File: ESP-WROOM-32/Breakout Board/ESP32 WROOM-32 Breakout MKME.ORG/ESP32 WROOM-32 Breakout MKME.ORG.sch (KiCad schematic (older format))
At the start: 1 part, among them U1 ESP32_DevKit_V1_DOIT

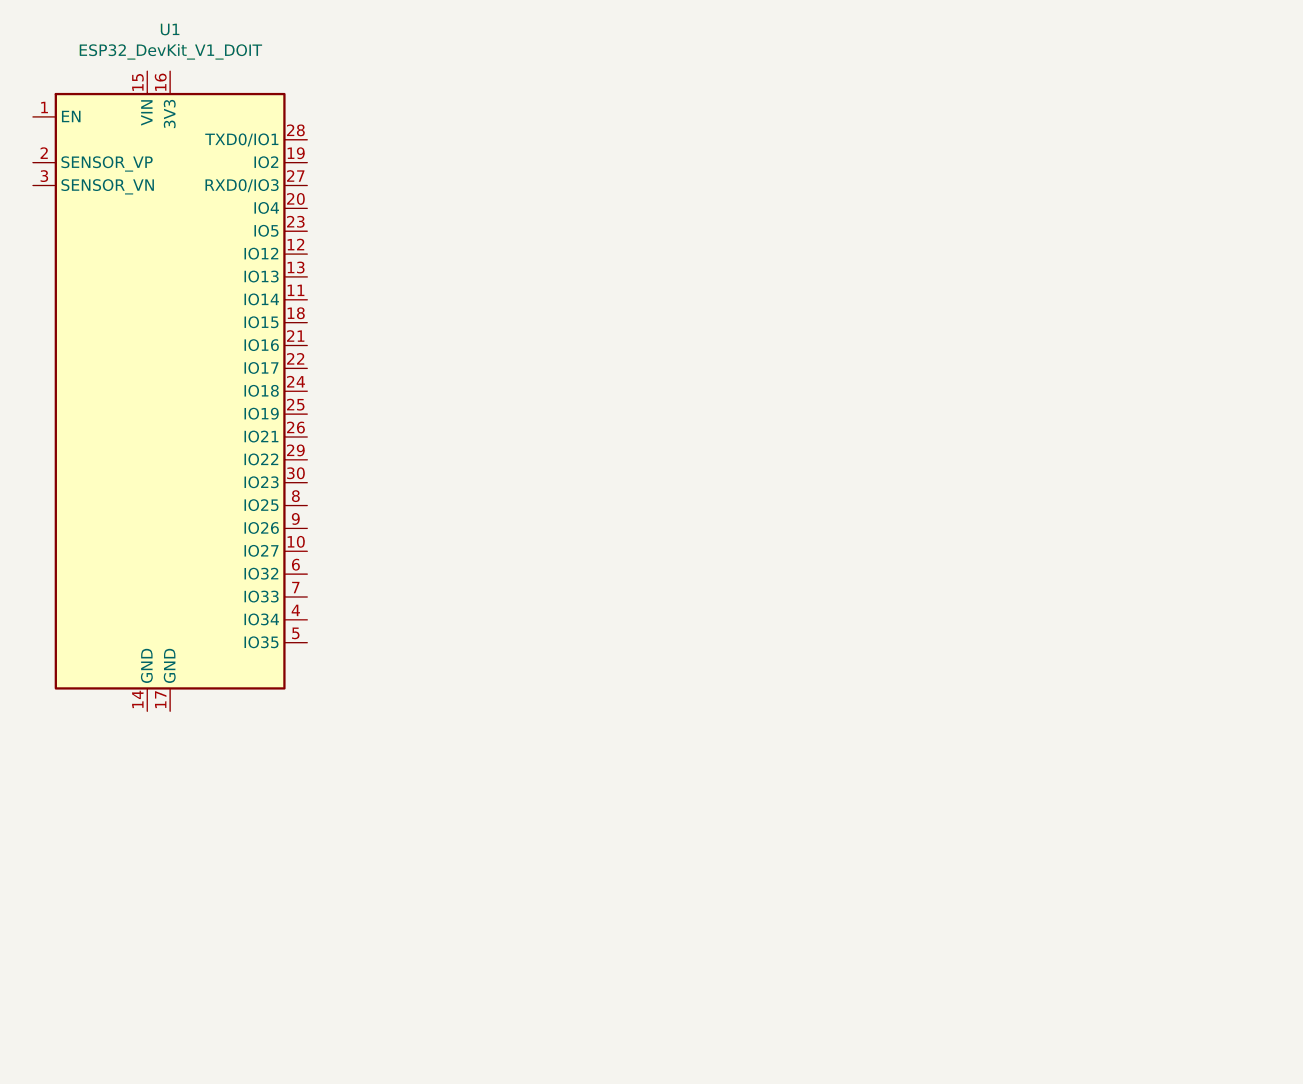
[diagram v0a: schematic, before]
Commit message: ref
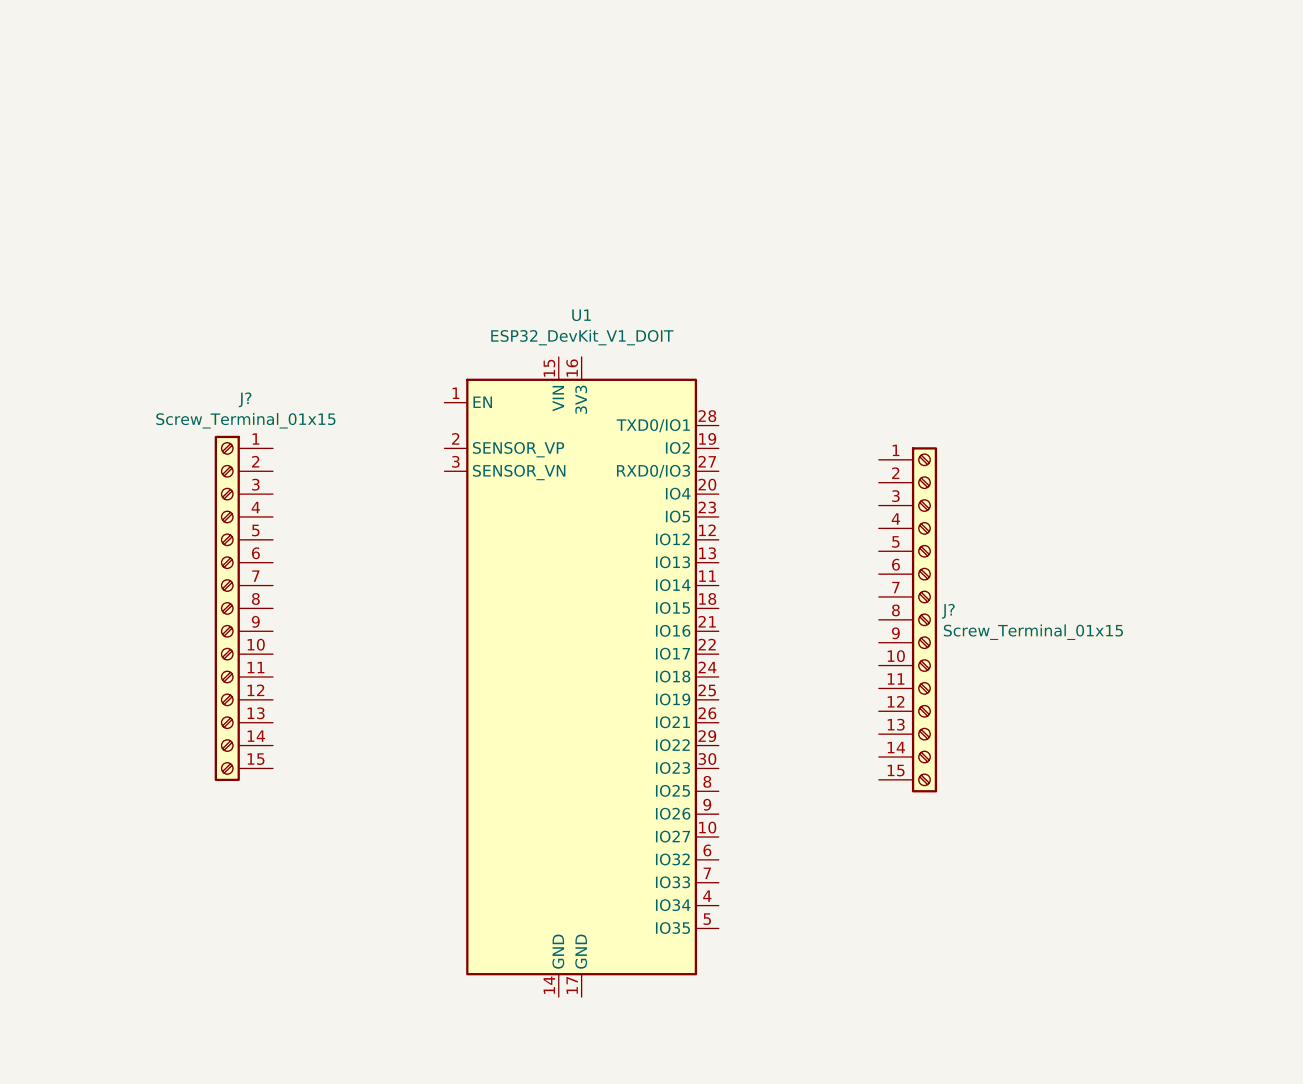
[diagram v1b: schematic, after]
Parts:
- added J? (x2): Screw_Terminal_01x15, symbol Connector:Screw_Terminal_01x15
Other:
- moved on the sheet: U1
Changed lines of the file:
@@
 L ESp3222:ESP32_DevKit_V1_DOIT U1
 U 1 1 6134E7FD
-P 6450 3350
-F 0 "U1" H 6450 4931 50  0000 C CNN
-F 1 "ESP32_DevKit_V1_DOIT" H 6450 4840 50  0000 C CNN
-F 2 "esp322:esp32_devkit_v1_doit" H 6000 4700 50  0001 C CNN
-F 3 "https://aliexpress.com/item/32864722159.html" H 6000 4700 50  0001 C CNN
-	1    6450 3350
+P 8250 4600
+F 0 "U1" H 8250 6181 50  0000 C CNN
+F 1 "ESP32_DevKit_V1_DOIT" H 8250 6090 50  0000 C CNN
+F 2 "esp322:esp32_devkit_v1_doit" H 7800 5950 50  0001 C CNN
+F 3 "https://aliexpress.com/item/32864722159.html" H 7800 5950 50  0001 C CNN
+	1    8250 4600
 	1    0    0    -1
 $EndComp
+$Comp
+L Connector:Screw_Terminal_01x15 J?
+U 1 1 61353EE6
+P 9750 4350
+F 0 "J?" H 9830 4392 50  0000 L CNN
+F 1 "Screw_Terminal_01x15" H 9830 4301 50  0000 L CNN
+F 2 "" H 9750 4350 50  0001 C CNN
+F 3 "~" H 9750 4350 50  0001 C CNN
+	1    9750 4350
+	1    0    0    -1
+$EndComp
+$Comp
+L Connector:Screw_Terminal_01x15 J?
+U 1 1 61354F94
+P 6700 4300
+F 0 "J?" H 6618 5217 50  0000 C CNN
+F 1 "Screw_Terminal_01x15" H 6618 5126 50  0000 C CNN
+F 2 "" H 6700 4300 50  0001 C CNN
+F 3 "~" H 6700 4300 50  0001 C CNN
+	1    6700 4300
+	-1   0    0    -1
+$EndComp
 $EndSCHEMATC

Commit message: Photos and kit updated
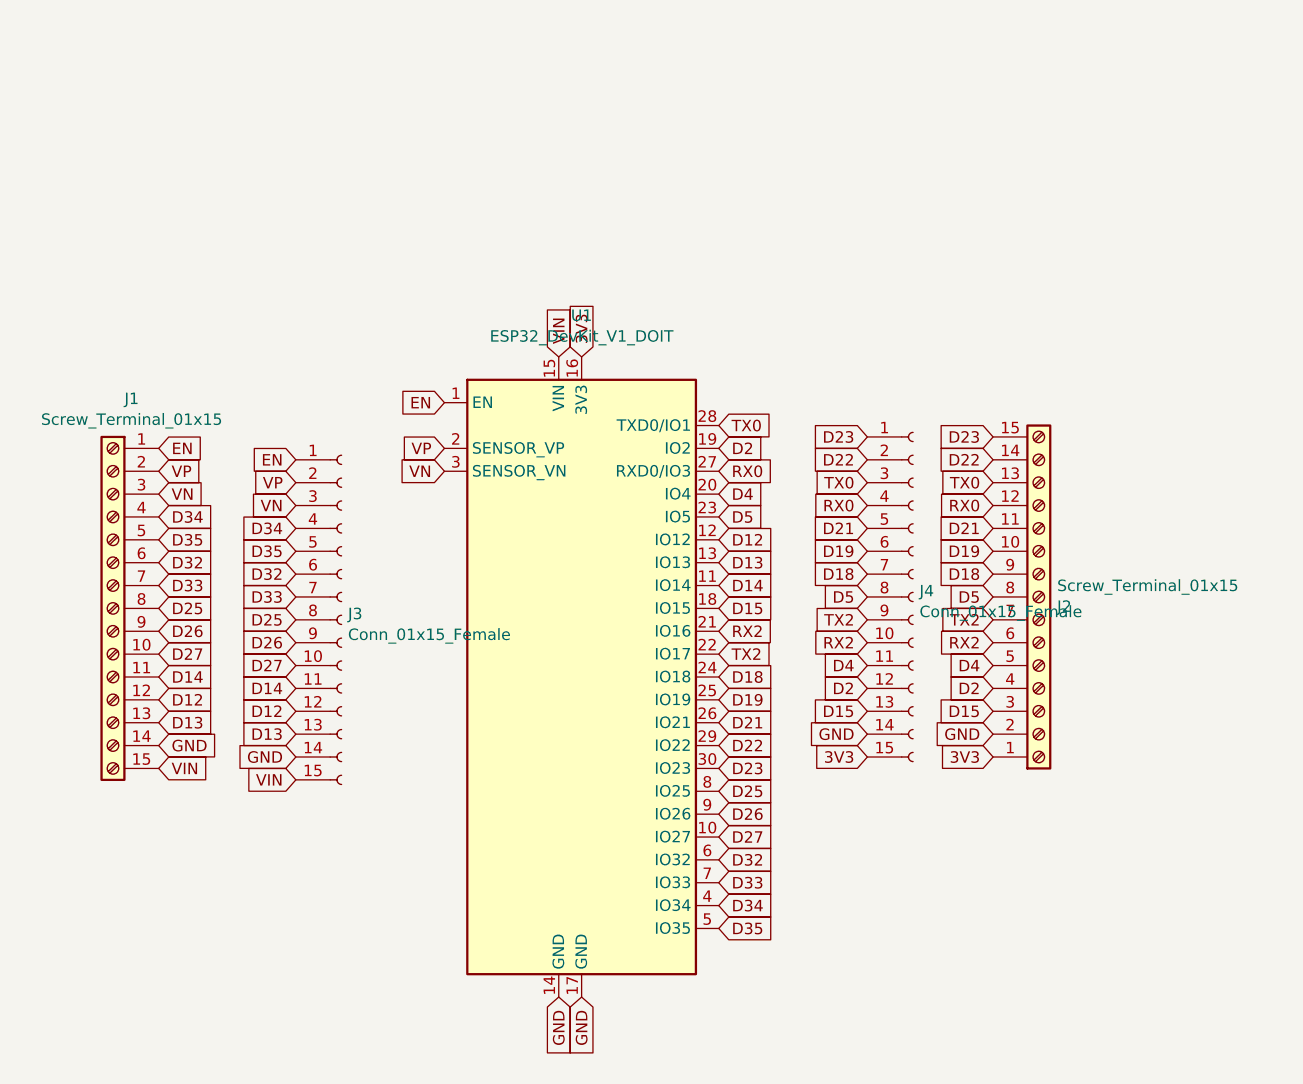
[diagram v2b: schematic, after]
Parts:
- added J3, J4: Conn_01x15_Female, Connector_PinHeader_2.54mm:PinHeader_1x15_P2.54mm_Vertical, symbol Connector:Conn_01x15_Female
- J1, J2: renamed from J?; footprint (none) -> TerminalBlock_Phoenix:TerminalBlock_Phoenix_MKDS-1,5-15-5.08_1x15_P5.08mm_Horizontal
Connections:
- net EN: now reaches U1.1 (EN)
- net EN: now also J1.1 (Pin_1), J3.1 (Pin_1)
- net D27: now reaches U1.10 (IO27)
- net D27: now also J1.10 (Pin_10), J3.10 (Pin_10)
- net D14: now reaches U1.11 (IO14)
- net D14: now also J1.11 (Pin_11), J3.11 (Pin_11)
- net D12: now reaches U1.12 (IO12)
- net D12: now also J1.12 (Pin_12), J3.12 (Pin_12)
- net D13: now reaches U1.13 (IO13)
- net D13: now also J1.13 (Pin_13), J3.13 (Pin_13)
- net GND: now reaches U1.14 (GND)
- net GND: now also J1.14 (Pin_14), J2.2 (Pin_2), U1.17 (GND), J3.14 (Pin_14), J4.14 (Pin_14)
- net VIN: now reaches U1.15 (VIN)
- net VIN: now also J1.15 (Pin_15), J3.15 (Pin_15)
- net 3V3: now reaches U1.16 (3V3)
- net 3V3: now also J2.1 (Pin_1), J4.15 (Pin_15)
- net D15: now reaches U1.18 (IO15)
- net D15: now also J2.3 (Pin_3), J4.13 (Pin_13)
- net D2: now reaches U1.19 (IO2)
- net D2: now also J2.4 (Pin_4), J4.12 (Pin_12)
- net VP: now reaches U1.2 (SENSOR_VP)
- net VP: now also J1.2 (Pin_2), J3.2 (Pin_2)
- net D4: now reaches U1.20 (IO4)
- net D4: now also J2.5 (Pin_5), J4.11 (Pin_11)
- net RX2: now reaches U1.21 (IO16)
- net RX2: now also J2.6 (Pin_6), J4.10 (Pin_10)
- net TX2: now reaches U1.22 (IO17)
- net TX2: now also J2.7 (Pin_7), J4.9 (Pin_9)
- net D5: now reaches U1.23 (IO5)
- net D5: now also J2.8 (Pin_8), J4.8 (Pin_8)
- net D18: now reaches U1.24 (IO18)
- net D18: now also J2.9 (Pin_9), J4.7 (Pin_7)
- net D19: now reaches U1.25 (IO19)
- net D19: now also J2.10 (Pin_10), J4.6 (Pin_6)
- net D21: now reaches U1.26 (IO21)
- net D21: now also J2.11 (Pin_11), J4.5 (Pin_5)
- net RX0: now reaches U1.27 (RXD0/IO3)
- net RX0: now also J2.12 (Pin_12), J4.4 (Pin_4)
- net TX0: now reaches U1.28 (TXD0/IO1)
- net TX0: now also J2.13 (Pin_13), J4.3 (Pin_3)
- net D22: now reaches U1.29 (IO22)
- net D22: now also J2.14 (Pin_14), J4.2 (Pin_2)
- net VN: now reaches U1.3 (SENSOR_VN)
- net VN: now also J1.3 (Pin_3), J3.3 (Pin_3)
- net D23: now reaches U1.30 (IO23)
- net D23: now also J2.15 (Pin_15), J4.1 (Pin_1)
- net D34: now reaches U1.4 (IO34)
- net D34: now also J1.4 (Pin_4), J3.4 (Pin_4)
- net D35: now reaches U1.5 (IO35)
- net D35: now also J1.5 (Pin_5), J3.5 (Pin_5)
- net D32: now reaches U1.6 (IO32)
- net D32: now also J1.6 (Pin_6), J3.6 (Pin_6)
- net D33: now reaches U1.7 (IO33)
- net D33: now also J1.7 (Pin_7), J3.7 (Pin_7)
- net D25: now reaches U1.8 (IO25)
- net D25: now also J1.8 (Pin_8), J3.8 (Pin_8)
- net D26: now reaches U1.9 (IO26)
- net D26: now also J1.9 (Pin_9), J3.9 (Pin_9)
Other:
- moved on the sheet: J1, J2
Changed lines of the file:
@@
 $EndDescr
+$Comp
+L Connector:Screw_Terminal_01x15 J2
+U 1 1 61353EE6
+P 10250 4250
+F 0 "J2" H 10330 4292 50  0000 L CNN
+F 1 "Screw_Terminal_01x15" H 10330 4201 50  0000 L CNN
+F 2 "TerminalBlock_Phoenix:TerminalBlock_Phoenix_MKDS-1,5-15-5.08_1x15_P5.08mm_Horizontal" H 10250 4250 50  0001 C CNN
+F 3 "~" H 10250 4250 50  0001 C CNN
+	1    10250 4250
+	1    0    0    1
+$EndComp
+$Comp
+L Connector:Screw_Terminal_01x15 J1
+U 1 1 61354F94
+P 6200 4300
+F 0 "J1" H 6118 5217 50  0000 C CNN
+F 1 "Screw_Terminal_01x15" H 6118 5126 50  0000 C CNN
+F 2 "TerminalBlock_Phoenix:TerminalBlock_Phoenix_MKDS-1,5-15-5.08_1x15_P5.08mm_Horizontal" H 6200 4300 50  0001 C CNN
+F 3 "~" H 6200 4300 50  0001 C CNN
+	1    6200 4300
+	-1   0    0    -1
+$EndComp
+Text GLabel 6400 3600 2    50   Input ~ 0
+EN
+Text GLabel 6400 3700 2    50   Input ~ 0
+VP
+Text GLabel 6400 4000 2    50   Input ~ 0
+D35
+Text GLabel 6400 3900 2    50   Input ~ 0
+D34
+Text GLabel 6400 4100 2    50   Input ~ 0
+D32
+Text GLabel 6400 4200 2    50   Input ~ 0
+D33
+Text GLabel 6400 4300 2    50   Input ~ 0
+D25
+Text GLabel 6400 4400 2    50   Input ~ 0
+D26
+Text GLabel 6400 4500 2    50   Input ~ 0
+D27
+Text GLabel 6400 4600 2    50   Input ~ 0
+D14
+Text GLabel 6400 4700 2    50   Input ~ 0
+D12
+Text GLabel 6400 4800 2    50   Input ~ 0
+D13
+Text GLabel 6400 4900 2    50   Input ~ 0
+GND
+Text GLabel 6400 5000 2    50   Input ~ 0
+VIN
+Text GLabel 6400 3800 2    50   Input ~ 0
+VN
+Text GLabel 7650 3400 0    50   Input ~ 0
+EN
+Text GLabel 8850 5700 2    50   Input ~ 0
+D35
+Text GLabel 8850 5600 2    50   Input ~ 0
+D34
+Text GLabel 8850 5400 2    50   Input ~ 0
+D32
+Text GLabel 8850 5500 2    50   Input ~ 0
+D33
+Text GLabel 8850 5100 2    50   Input ~ 0
+D25
+Text GLabel 8850 5200 2    50   Input ~ 0
+D26
+Text GLabel 8850 5300 2    50   Input ~ 0
+D27
+Text GLabel 8850 4200 2    50   Input ~ 0
+D14
+Text GLabel 8850 4000 2    50   Input ~ 0
+D12
+Text GLabel 8850 4100 2    50   Input ~ 0
+D13
+Text GLabel 8150 6000 3    50   Input ~ 0
+GND
+Text GLabel 8150 3200 1    50   Input ~ 0
+VIN
+Text GLabel 7650 3700 0    50   Input ~ 0
+VN
+Text GLabel 10050 3550 0    50   Input ~ 0
+D23
+Text GLabel 10050 3650 0    50   Input ~ 0
+D22
+Text GLabel 10050 3750 0    50   Input ~ 0
+TX0
+Text GLabel 10050 3850 0    50   Input ~ 0
+RX0
+Text GLabel 10050 3950 0    50   Input ~ 0
+D21
+Text GLabel 10050 4050 0    50   Input ~ 0
+D19
+Text GLabel 10050 4150 0    50   Input ~ 0
+D18
+Text GLabel 10050 4250 0    50   Input ~ 0
+D5
+Text GLabel 10050 4350 0    50   Input ~ 0
+TX2
+Text GLabel 10050 4450 0    50   Input ~ 0
+RX2
+Text GLabel 10050 4550 0    50   Input ~ 0
+D4
+Text GLabel 10050 4650 0    50   Input ~ 0
+D2
+Text GLabel 10050 4750 0    50   Input ~ 0
+D15
+Text GLabel 10050 4850 0    50   Input ~ 0
+GND
+Text GLabel 10050 4950 0    50   Input ~ 0
+3V3
+Text GLabel 8850 5000 2    50   Input ~ 0
+D23
+Text GLabel 8850 4900 2    50   Input ~ 0
+D22
+Text GLabel 8850 3500 2    50   Input ~ 0
+TX0
+Text GLabel 8850 3700 2    50   Input ~ 0
+RX0
+Text GLabel 8850 4800 2    50   Input ~ 0
+D21
+Text GLabel 8850 4700 2    50   Input ~ 0
+D19
+Text GLabel 8850 4600 2    50   Input ~ 0
+D18
+Text GLabel 8850 3900 2    50   Input ~ 0
+D5
+Text GLabel 8850 4500 2    50   Input ~ 0
+TX2
+Text GLabel 8850 4400 2    50   Input ~ 0
+RX2
+Text GLabel 8850 3800 2    50   Input ~ 0
+D4
+Text GLabel 8850 3600 2    50   Input ~ 0
+D2
+Text GLabel 8850 4300 2    50   Input ~ 0
+D15
+Text GLabel 8250 6000 3    50   Input ~ 0
+GND
+Text GLabel 8250 3200 1    50   Input ~ 0
+3V3
+Text GLabel 7650 3600 0    50   Input ~ 0
+VP
 $Comp
 L ESp3222:ESP32_DevKit_V1_DOIT U1
@@
 $EndComp
 $Comp
-L Connector:Screw_Terminal_01x15 J?
-U 1 1 61353EE6
-P 9750 4350
-F 0 "J?" H 9830 4392 50  0000 L CNN
-F 1 "Screw_Terminal_01x15" H 9830 4301 50  0000 L CNN
-F 2 "" H 9750 4350 50  0001 C CNN
-F 3 "~" H 9750 4350 50  0001 C CNN
-	1    9750 4350
+L Connector:Conn_01x15_Female J3
+U 1 1 615E00ED
+P 7200 4350
+F 0 "J3" H 7228 4376 50  0000 L CNN
+F 1 "Conn_01x15_Female" H 7228 4285 50  0000 L CNN
+F 2 "Connector_PinHeader_2.54mm:PinHeader_1x15_P2.54mm_Vertical" H 7200 4350 50  0001 C CNN
+F 3 "~" H 7200 4350 50  0001 C CNN
+	1    7200 4350
 	1    0    0    -1
 $EndComp
 $Comp
-L Connector:Screw_Terminal_01x15 J?
-U 1 1 61354F94
-P 6700 4300
-F 0 "J?" H 6618 5217 50  0000 C CNN
-F 1 "Screw_Terminal_01x15" H 6618 5126 50  0000 C CNN
-F 2 "" H 6700 4300 50  0001 C CNN
-F 3 "~" H 6700 4300 50  0001 C CNN
-	1    6700 4300
-	-1   0    0    -1
-$EndComp
+L Connector:Conn_01x15_Female J4
+U 1 1 615E1469
+P 9700 4250
+F 0 "J4" H 9728 4276 50  0000 L CNN
+F 1 "Conn_01x15_Female" H 9728 4185 50  0000 L CNN
+F 2 "Connector_PinHeader_2.54mm:PinHeader_1x15_P2.54mm_Vertical" H 9700 4250 50  0001 C CNN
+F 3 "~" H 9700 4250 50  0001 C CNN
+	1    9700 4250
+	1    0    0    -1
+$EndComp
+Text GLabel 7000 4950 0    50   Input ~ 0
+GND
+Text GLabel 7000 5050 0    50   Input ~ 0
+VIN
+Text GLabel 7000 3850 0    50   Input ~ 0
+VN
+Text GLabel 7000 4850 0    50   Input ~ 0
+D13
+Text GLabel 7000 4750 0    50   Input ~ 0
+D12
+Text GLabel 7000 4650 0    50   Input ~ 0
+D14
+Text GLabel 7000 4550 0    50   Input ~ 0
+D27
+Text GLabel 7000 4450 0    50   Input ~ 0
+D26
+Text GLabel 7000 4350 0    50   Input ~ 0
+D25
+Text GLabel 7000 4250 0    50   Input ~ 0
+D33
+Text GLabel 7000 4150 0    50   Input ~ 0
+D32
+Text GLabel 7000 3950 0    50   Input ~ 0
+D34
+Text GLabel 7000 4050 0    50   Input ~ 0
+D35
+Text GLabel 7000 3750 0    50   Input ~ 0
+VP
+Text GLabel 7000 3650 0    50   Input ~ 0
+EN
+Text GLabel 9500 3550 0    50   Input ~ 0
+D23
+Text GLabel 9500 3650 0    50   Input ~ 0
+D22
+Text GLabel 9500 3750 0    50   Input ~ 0
+TX0
+Text GLabel 9500 3850 0    50   Input ~ 0
+RX0
+Text GLabel 9500 3950 0    50   Input ~ 0
+D21
+Text GLabel 9500 4050 0    50   Input ~ 0
+D19
+Text GLabel 9500 4150 0    50   Input ~ 0
+D18
+Text GLabel 9500 4250 0    50   Input ~ 0
+D5
+Text GLabel 9500 4350 0    50   Input ~ 0
+TX2
+Text GLabel 9500 4450 0    50   Input ~ 0
+RX2
+Text GLabel 9500 4550 0    50   Input ~ 0
+D4
+Text GLabel 9500 4650 0    50   Input ~ 0
+D2
+Text GLabel 9500 4750 0    50   Input ~ 0
+D15
+Text GLabel 9500 4850 0    50   Input ~ 0
+GND
+Text GLabel 9500 4950 0    50   Input ~ 0
+3V3
 $EndSCHEMATC

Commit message: Breakout board DONE
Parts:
- J1: footprint TerminalBlock_Phoenix:TerminalBlock_Phoenix_MKDS-1,5-15-5.08_1x15_P5.08mm_Horizontal -> TerminalBlock_Phoenix:TerminalBlock_Phoenix_MKDS-1,5-16-5.08_1x16_P5.08mm_Horizontal
- J2: footprint TerminalBlock_Phoenix:TerminalBlock_Phoenix_MKDS-1,5-15-5.08_1x15_P5.08mm_Horizontal -> TerminalBlock_Phoenix:TerminalBlock_Phoenix_MKDS-1,5-16-5.08_1x16_P5.08mm_Horizontal; symbol Connector:Screw_Terminal_01x15 -> Connector:Screw_Terminal_01x16
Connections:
- net 3V3: now also J2.2 (Pin_2); no longer J2.1 (Pin_1)
- net D15: now also J2.4 (Pin_4); no longer J2.3 (Pin_3)
- net D18: now also J2.10 (Pin_10); no longer J2.9 (Pin_9)
- net D19: now also J2.11 (Pin_11); no longer J2.10 (Pin_10)
- net D2: now also J2.5 (Pin_5); no longer J2.4 (Pin_4)
- net D21: now also J2.12 (Pin_12); no longer J2.11 (Pin_11)
- net D22: now also J2.15 (Pin_15); no longer J2.14 (Pin_14)
- net D23: now also J2.16 (Pin_16); no longer J2.15 (Pin_15)
- net D4: now also J2.6 (Pin_6); no longer J2.5 (Pin_5)
- net D5: now also J2.9 (Pin_9); no longer J2.8 (Pin_8)
- net GND: now also J2.3 (Pin_3); no longer J2.2 (Pin_2)
- net RX0: now also J2.13 (Pin_13); no longer J2.12 (Pin_12)
- net RX2: now also J2.7 (Pin_7); no longer J2.6 (Pin_6)
- net TX0: now also J2.14 (Pin_14); no longer J2.13 (Pin_13)
- net TX2: now also J2.8 (Pin_8); no longer J2.7 (Pin_7)
- no-connect marks 0 -> 1
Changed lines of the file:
@@
 $EndDescr
-$Comp
-L Connector:Screw_Terminal_01x15 J2
-U 1 1 61353EE6
-P 10250 4250
-F 0 "J2" H 10330 4292 50  0000 L CNN
-F 1 "Screw_Terminal_01x15" H 10330 4201 50  0000 L CNN
-F 2 "TerminalBlock_Phoenix:TerminalBlock_Phoenix_MKDS-1,5-15-5.08_1x15_P5.08mm_Horizontal" H 10250 4250 50  0001 C CNN
-F 3 "~" H 10250 4250 50  0001 C CNN
-	1    10250 4250
-	1    0    0    1
-$EndComp
 $Comp
 L Connector:Screw_Terminal_01x15 J1
@@
 F 0 "J1" H 6118 5217 50  0000 C CNN
 F 1 "Screw_Terminal_01x15" H 6118 5126 50  0000 C CNN
-F 2 "TerminalBlock_Phoenix:TerminalBlock_Phoenix_MKDS-1,5-15-5.08_1x15_P5.08mm_Horizontal" H 6200 4300 50  0001 C CNN
+F 2 "TerminalBlock_Phoenix:TerminalBlock_Phoenix_MKDS-1,5-16-5.08_1x16_P5.08mm_Horizontal" H 6200 4300 50  0001 C CNN
 F 3 "~" H 6200 4300 50  0001 C CNN
 	1    6200 4300
@@
 Text GLabel 7650 3700 0    50   Input ~ 0
 VN
+Text GLabel 10050 3450 0    50   Input ~ 0
+D23
 Text GLabel 10050 3550 0    50   Input ~ 0
-D23
+D22
 Text GLabel 10050 3650 0    50   Input ~ 0
-D22
+TX0
 Text GLabel 10050 3750 0    50   Input ~ 0
-TX0
+RX0
 Text GLabel 10050 3850 0    50   Input ~ 0
-RX0
+D21
 Text GLabel 10050 3950 0    50   Input ~ 0
-D21
+D19
 Text GLabel 10050 4050 0    50   Input ~ 0
-D19
+D18
 Text GLabel 10050 4150 0    50   Input ~ 0
-D18
+D5
 Text GLabel 10050 4250 0    50   Input ~ 0
-D5
+TX2
 Text GLabel 10050 4350 0    50   Input ~ 0
-TX2
+RX2
 Text GLabel 10050 4450 0    50   Input ~ 0
-RX2
+D4
 Text GLabel 10050 4550 0    50   Input ~ 0
-D4
+D2
 Text GLabel 10050 4650 0    50   Input ~ 0
-D2
+D15
 Text GLabel 10050 4750 0    50   Input ~ 0
-D15
+GND
 Text GLabel 10050 4850 0    50   Input ~ 0
-GND
-Text GLabel 10050 4950 0    50   Input ~ 0
 3V3
 Text GLabel 8850 5000 2    50   Input ~ 0
@@
 Text GLabel 9500 4950 0    50   Input ~ 0
 3V3
+$Comp
+L Connector:Screw_Terminal_01x16 J2
+U 1 1 61353EE6
+P 10250 4250
+F 0 "J2" H 10330 4292 50  0000 L CNN
+F 1 "Screw_Terminal_01x15" H 10330 4201 50  0000 L CNN
+F 2 "TerminalBlock_Phoenix:TerminalBlock_Phoenix_MKDS-1,5-16-5.08_1x16_P5.08mm_Horizontal" H 10250 4250 50  0001 C CNN
+F 3 "~" H 10250 4250 50  0001 C CNN
+	1    10250 4250
+	1    0    0    1
+$EndComp
+NoConn ~ 10050 4950
 $EndSCHEMATC
